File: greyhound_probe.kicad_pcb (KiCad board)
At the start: 2 copper layers, 40 parts, among them J1 USB_C_Receptacle_USB2.0, J2 Conn_01x04_Male, J3 FTSH-105-01-L-DV-K-TR, Q1 IRLML6401, SW1 SW_SPDT, U1 XC6206P332MR, U2 USBLC6-2SC6, U3 STM32F072CBUx

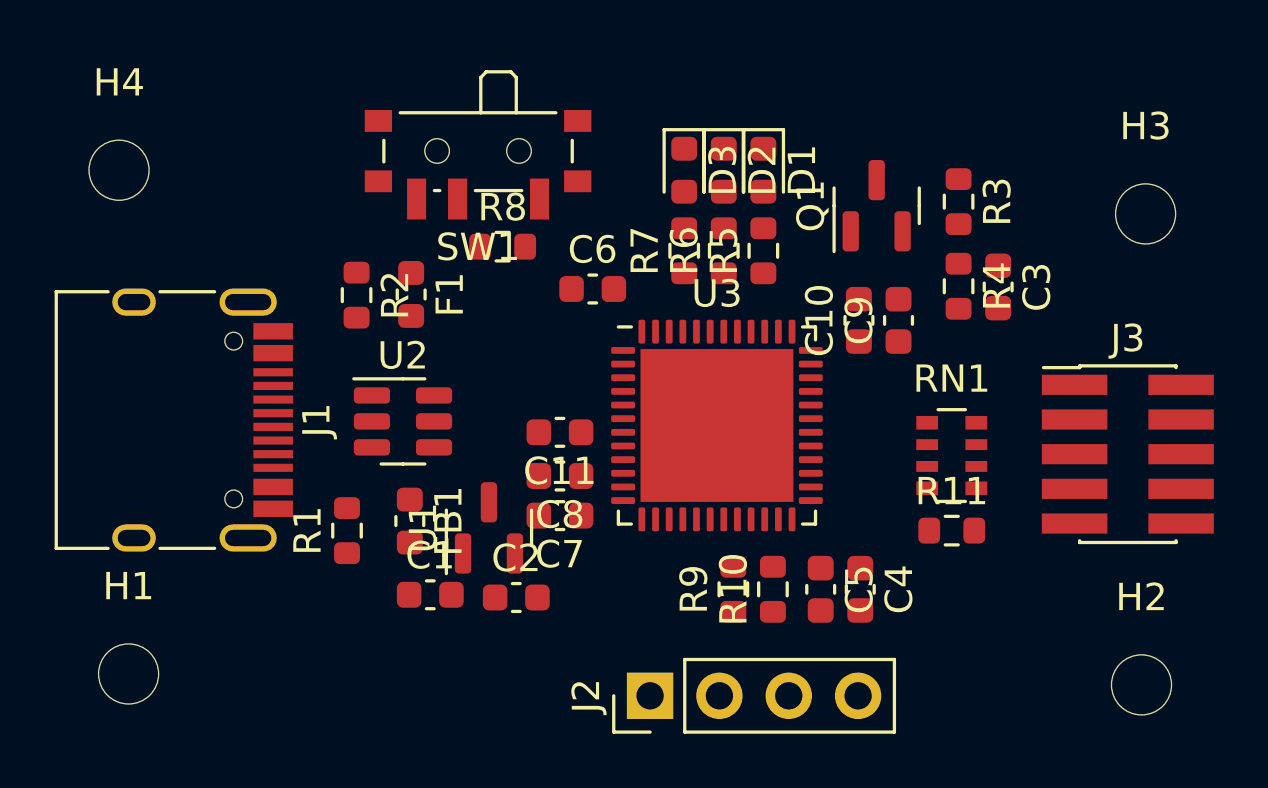
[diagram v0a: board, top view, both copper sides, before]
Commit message: Fixed short and power symbols
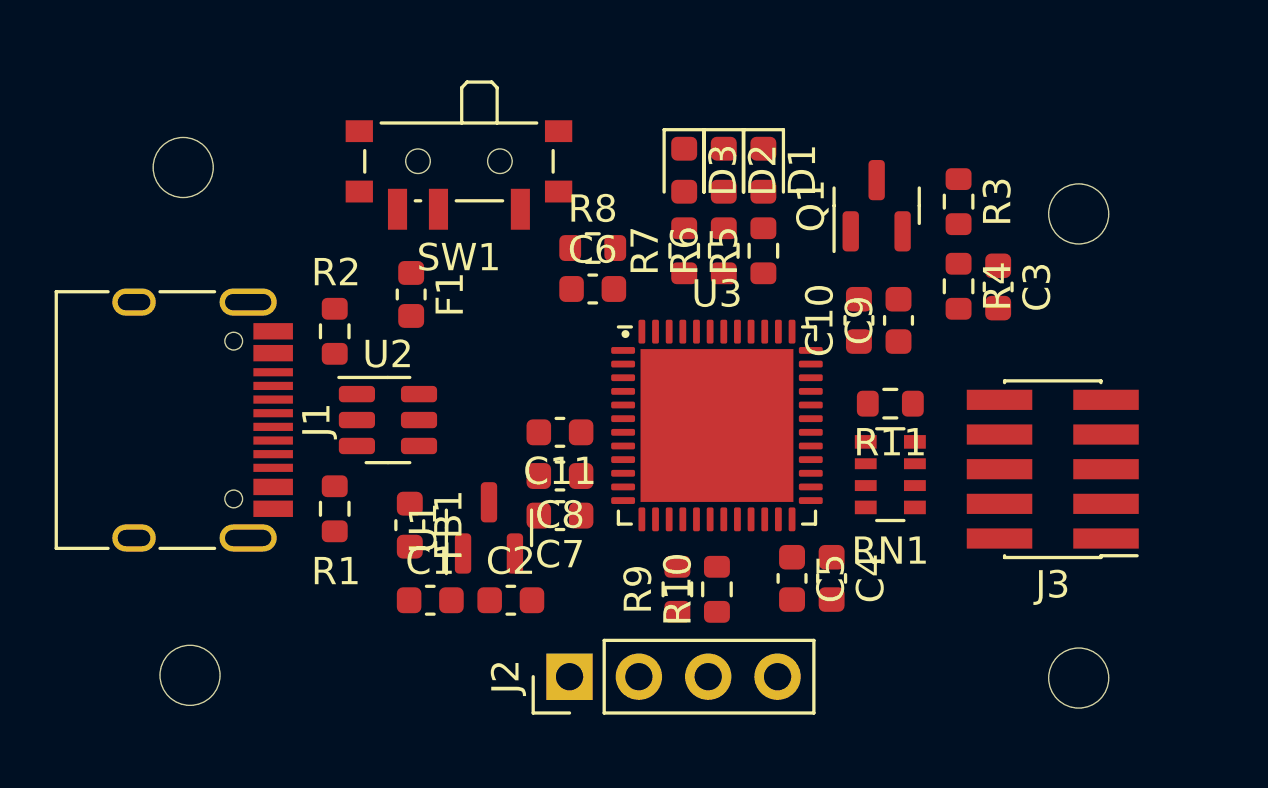
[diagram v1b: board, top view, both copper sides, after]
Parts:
- moved R11 5.17 mm to (148.6, 77.5), turned to 180 degrees
- moved R8 3.30 mm to (137.7, 71.8)
- moved J2 3.03 mm to (136.8, 87.5)
- moved J3 2.80 mm to (154.5, 79.8), turned to 180 degrees
- moved H3 2.45 mm to (155.4, 70.5)
- moved RN1 2.36 mm to (148.6, 80.0), turned to 180 degrees
- moved H4 2.35 mm to (122.7, 68.8)
- moved H2 2.31 mm to (155.4, 87.5)
- moved H1 2.25 mm to (122.9, 87.4)
- moved R10 2.05 mm to (142.2, 84.2)
- moved R9 2.05 mm to (140.8, 84.2)
- moved R2 1.55 mm to (128.2, 74.8)
- moved C5 1.12 mm to (144.9, 83.8)
- moved C4 1.12 mm to (146.4, 83.8)
- moved R1 0.92 mm to (128.2, 81.3)
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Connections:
- C1 pad 2: +3.3V -> GND
- C10 pad 2: +3.3V -> GND
- C11 pad 2: +3.3V -> GND
- C2 pad 2: +3.3V -> GND
- C3 pad 2: +3.3V -> GND
- C4 pad 2: +3.3V -> GND
- C5 pad 2: +3.3V -> GND
- C6 pad 2: +3.3V -> GND
- C7 pad 2: +3.3V -> GND
- C8 pad 2: +3.3V -> GND
- C9 pad 2: +3.3V -> GND
- D1 pad 1: +3.3V -> GND
- D2 pad 1: +3.3V -> GND
- D3 pad 1: +3.3V -> GND
- J1 pad A1: +3.3V -> GND
- J1 pad A12: +3.3V -> GND
- J1 pad B1: +3.3V -> GND
- J1 pad B12: +3.3V -> GND
- J2 pad 4: +3.3V -> GND
- J3 pad 3: +3.3V -> GND
- J3 pad 5: +3.3V -> GND
- J3 pad 9: +3.3V -> GND
- R1 pad 1: +3.3V -> GND
- R2 pad 1: +3.3V -> GND
- R4 pad 2: +3.3V -> GND
- SW1 pad 1: +3.3V -> GND
- U1 pad 1: +3.3V -> GND
- U2 pad 2: +3.3V -> GND
- U3 pad 23: +3.3V -> GND
- U3 pad 25: /TARGET_TDO -> /TARGET_TCK
- U3 pad 26: /TARGET_TCK -> /TARGET_TMS
- U3 pad 27: /TARGET_TMS -> /TARGET_TDO
- U3 pad 35: +3.3V -> GND
- U3 pad 47: +3.3V -> GND
- U3 pad 49: +3.3V -> GND
- U3 pad 8: +3.3V -> GND
